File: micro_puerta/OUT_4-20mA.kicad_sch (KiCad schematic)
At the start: 2 parts

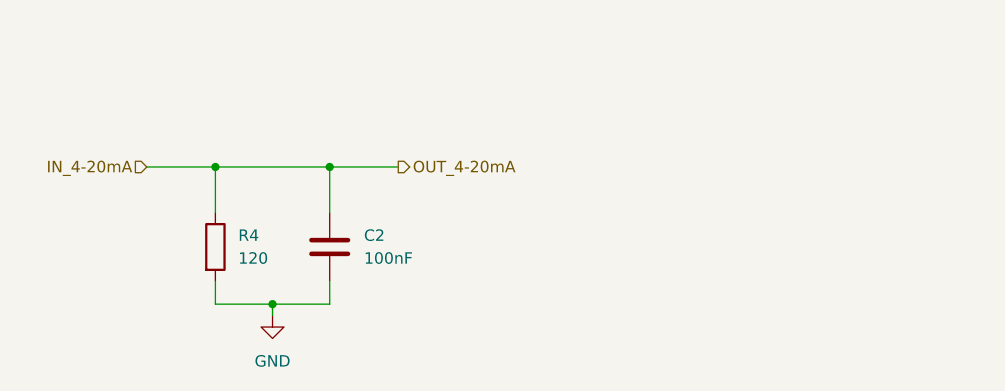
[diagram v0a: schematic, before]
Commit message: actualizacion placa
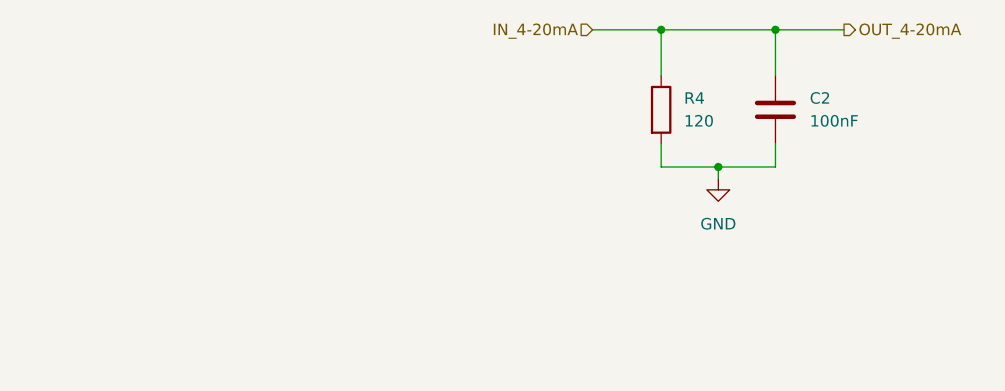
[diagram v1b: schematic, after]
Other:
- moved on the sheet: C2, R4
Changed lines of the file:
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@@
 	(paper "A4")
 	(junction
-		(at 97.79 115.57)
+		(at 147.32 100.33)
 		(diameter 0)
 		(color 0 0 0 0)
 	)
 	(junction
-		(at 91.44 100.33)
+		(at 140.97 85.09)
 		(diameter 0)
 		(color 0 0 0 0)
 	)
 	(junction
-		(at 104.14 100.33)
+		(at 153.67 85.09)
 		(diameter 0)
 		(color 0 0 0 0)
@@
 	(wire
 		(pts
-			(xy 83.82 100.33) (xy 91.44 100.33)
-		)
-		(stroke
-			(width 0)
-			(type default)
-		)
-	)
-	(wire
-		(pts
-			(xy 91.44 100.33) (xy 104.14 100.33)
-		)
-		(stroke
-			(width 0)
-			(type default)
-		)
-	)
-	(wire
-		(pts
-			(xy 104.14 115.57) (xy 97.79 115.57)
-		)
-		(stroke
-			(width 0)
-			(type default)
-		)
-	)
-	(wire
-		(pts
-			(xy 97.79 115.57) (xy 91.44 115.57)
-		)
-		(stroke
-			(width 0)
-			(type default)
-		)
-	)
-	(wire
-		(pts
-			(xy 104.14 100.33) (xy 104.14 105.41)
-		)
-		(stroke
-			(width 0)
-			(type default)
-		)
-	)
-	(wire
-		(pts
-			(xy 97.79 115.57) (xy 97.79 116.84)
-		)
-		(stroke
-			(width 0)
-			(type default)
-		)
-	)
-	(wire
-		(pts
-			(xy 104.14 113.03) (xy 104.14 115.57)
-		)
-		(stroke
-			(width 0)
-			(type default)
-		)
-	)
-	(wire
-		(pts
-			(xy 91.44 115.57) (xy 91.44 113.03)
-		)
-		(stroke
-			(width 0)
-			(type default)
-		)
-	)
-	(wire
-		(pts
-			(xy 104.14 100.33) (xy 111.76 100.33)
-		)
-		(stroke
-			(width 0)
-			(type default)
-		)
-	)
-	(wire
-		(pts
-			(xy 91.44 100.33) (xy 91.44 105.41)
+			(xy 133.35 85.09) (xy 140.97 85.09)
+		)
+		(stroke
+			(width 0)
+			(type default)
+		)
+	)
+	(wire
+		(pts
+			(xy 140.97 85.09) (xy 153.67 85.09)
+		)
+		(stroke
+			(width 0)
+			(type default)
+		)
+	)
+	(wire
+		(pts
+			(xy 153.67 100.33) (xy 147.32 100.33)
+		)
+		(stroke
+			(width 0)
+			(type default)
+		)
+	)
+	(wire
+		(pts
+			(xy 147.32 100.33) (xy 140.97 100.33)
+		)
+		(stroke
+			(width 0)
+			(type default)
+		)
+	)
+	(wire
+		(pts
+			(xy 153.67 85.09) (xy 153.67 90.17)
+		)
+		(stroke
+			(width 0)
+			(type default)
+		)
+	)
+	(wire
+		(pts
+			(xy 147.32 100.33) (xy 147.32 101.6)
+		)
+		(stroke
+			(width 0)
+			(type default)
+		)
+	)
+	(wire
+		(pts
+			(xy 153.67 97.79) (xy 153.67 100.33)
+		)
+		(stroke
+			(width 0)
+			(type default)
+		)
+	)
+	(wire
+		(pts
+			(xy 140.97 100.33) (xy 140.97 97.79)
+		)
+		(stroke
+			(width 0)
+			(type default)
+		)
+	)
+	(wire
+		(pts
+			(xy 153.67 85.09) (xy 161.29 85.09)
+		)
+		(stroke
+			(width 0)
+			(type default)
+		)
+	)
+	(wire
+		(pts
+			(xy 140.97 85.09) (xy 140.97 90.17)
 		)
 		(stroke
@@
 	(hierarchical_label "IN_4-20mA"
 		(shape input)
-		(at 83.82 100.33 180)
+		(at 133.35 85.09 180)
 		(effects
 			(font
@@
 	(hierarchical_label "OUT_4-20mA"
 		(shape output)
-		(at 111.76 100.33 0)
+		(at 161.29 85.09 0)
 		(effects
 			(font
@@
 	(symbol
 		(lib_id "power:GND")
-		(at 97.79 116.84 0)
+		(at 147.32 101.6 0)
 		(unit 1)
 		(exclude_from_sim no)
@@
 		(fields_autoplaced yes)
 		(property "Reference" "#PWR016"
-			(at 97.79 123.19 0)
+			(at 147.32 107.95 0)
 			(effects
 				(font
@@
 		)
 		(property "Value" "GND"
-			(at 97.79 121.92 0)
+			(at 147.32 106.68 0)
 			(effects
 				(font
@@
 		)
 		(property "Footprint" ""
-			(at 97.79 116.84 0)
+			(at 147.32 101.6 0)
 			(effects
 				(font
@@
 		)
 		(property "Datasheet" ""
-			(at 97.79 116.84 0)
+			(at 147.32 101.6 0)
 			(effects
 				(font
@@
 		)
 		(property "Description" "Power symbol creates a global label with name \"GND\" , ground"
-			(at 97.79 116.84 0)
+			(at 147.32 101.6 0)
 			(effects
 				(font
@@
 	(symbol
 		(lib_id "Device:C")
-		(at 104.14 109.22 0)
+		(at 153.67 93.98 0)
 		(unit 1)
 		(exclude_from_sim no)
@@
 		(fields_autoplaced yes)
 		(property "Reference" "C2"
-			(at 107.95 107.9499 0)
+			(at 157.48 92.7099 0)
 			(effects
 				(font
@@
 		)
 		(property "Value" "100nF"
-			(at 107.95 110.4899 0)
+			(at 157.48 95.2499 0)
 			(effects
 				(font
@@
 		)
 		(property "Footprint" ""
-			(at 105.1052 113.03 0)
+			(at 154.6352 97.79 0)
 			(effects
 				(font
@@
 		)
 		(property "Datasheet" "~"
-			(at 104.14 109.22 0)
+			(at 153.67 93.98 0)
 			(effects
 				(font
@@
 		)
 		(property "Description" "Unpolarized capacitor"
-			(at 104.14 109.22 0)
+			(at 153.67 93.98 0)
 			(effects
 				(font
@@
 	(symbol
 		(lib_id "Device:R")
-		(at 91.44 109.22 0)
+		(at 140.97 93.98 0)
 		(unit 1)
 		(exclude_from_sim no)
@@
 		(fields_autoplaced yes)
 		(property "Reference" "R4"
-			(at 93.98 107.9499 0)
+			(at 143.51 92.7099 0)
 			(effects
 				(font
@@
 		)
 		(property "Value" "120"
-			(at 93.98 110.4899 0)
+			(at 143.51 95.2499 0)
 			(effects
 				(font
@@
 		)
 		(property "Footprint" ""
-			(at 89.662 109.22 90)
+			(at 139.192 93.98 90)
 			(effects
 				(font
@@
 		)
 		(property "Datasheet" "~"
-			(at 91.44 109.22 0)
+			(at 140.97 93.98 0)
 			(effects
 				(font
@@
 		)
 		(property "Description" "Resistor"
-			(at 91.44 109.22 0)
-			(effects
-				(font
+			(at 140.97 93.98 0)
+			(effects
+				(font
